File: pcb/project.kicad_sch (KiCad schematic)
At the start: 5 parts, among them J1 USB_B_Micro, U1 RP2040, U2 NCP1117-3.3_SOT223

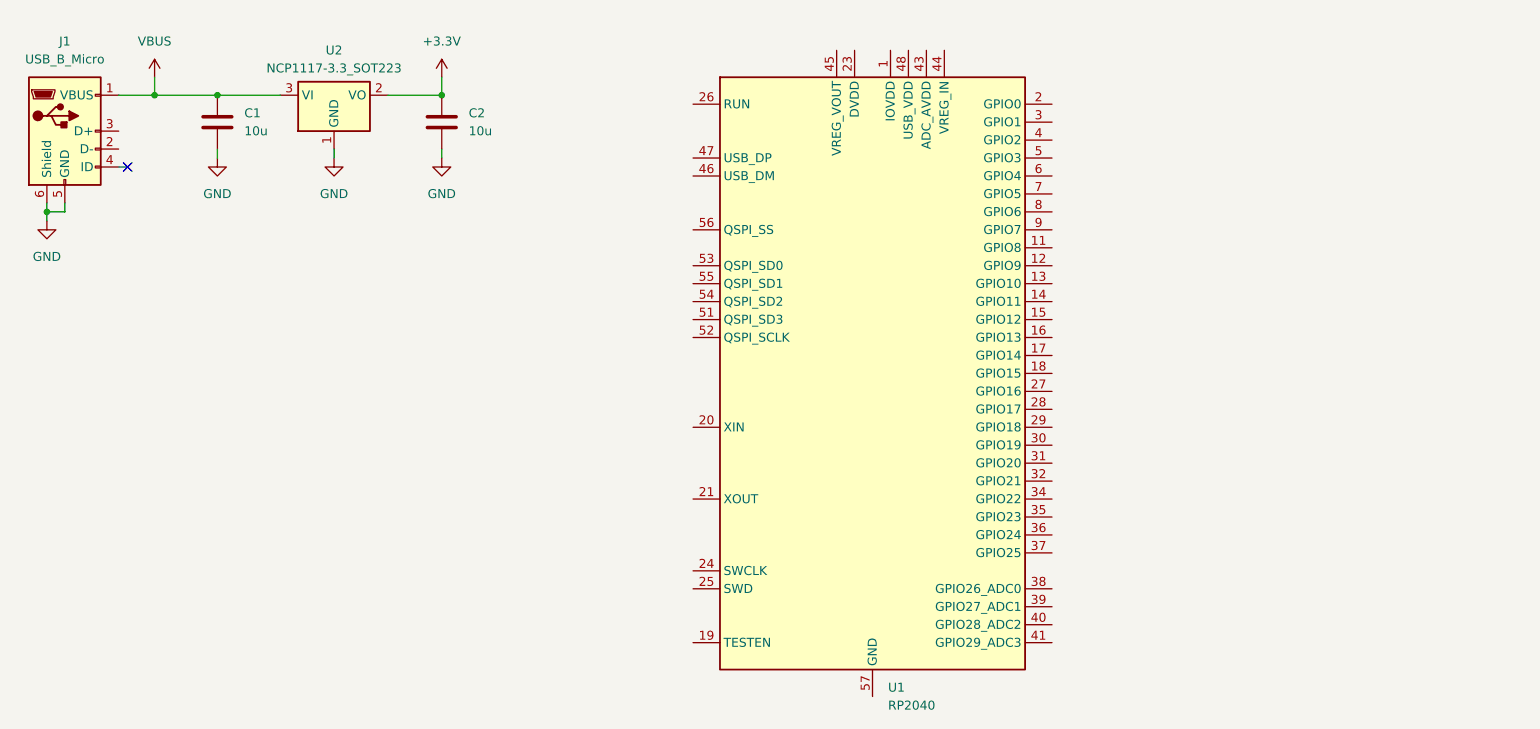
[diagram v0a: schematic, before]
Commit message: Implemented circuit
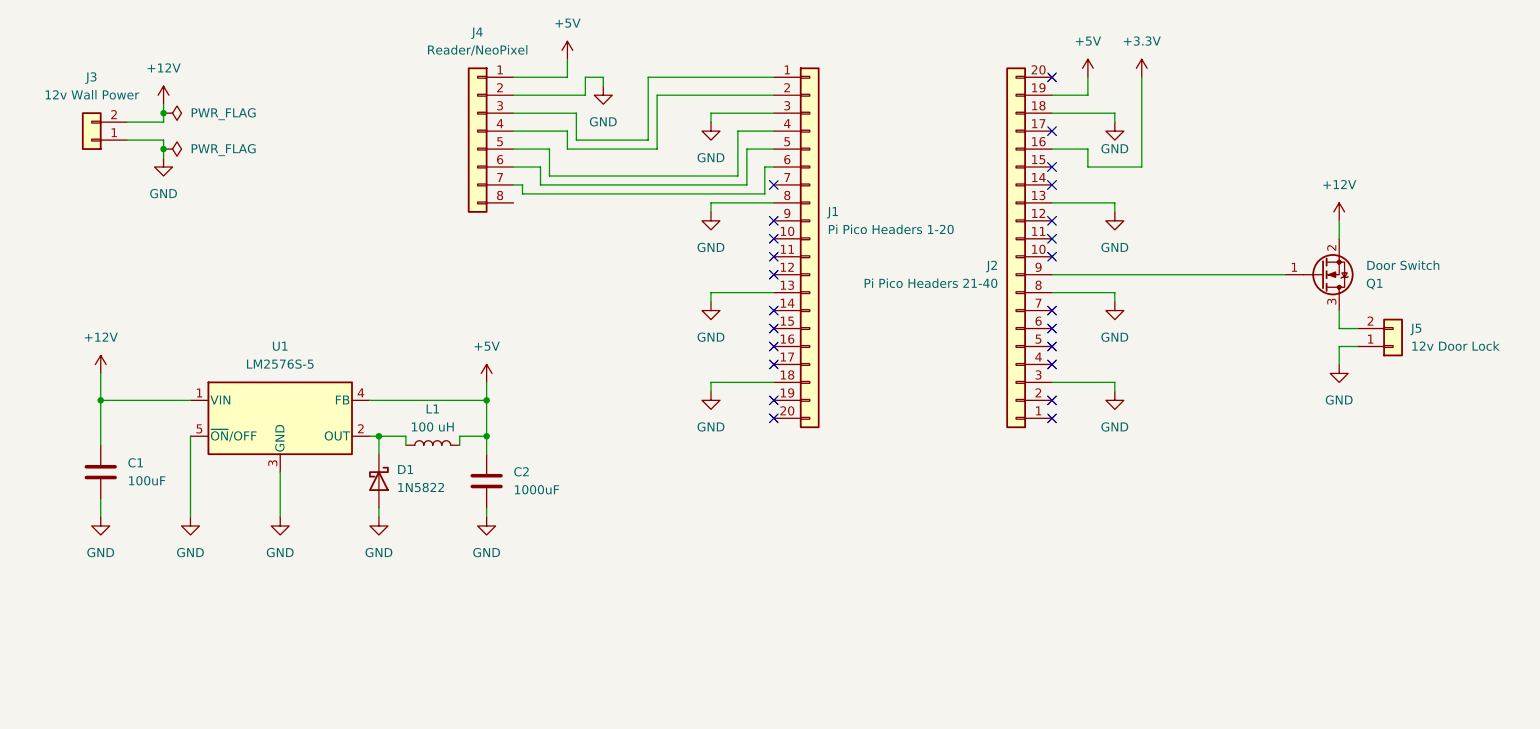
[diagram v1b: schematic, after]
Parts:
- removed J1: USB_B_Micro, symbol Connector:USB_B_Micro
- removed U1: RP2040, Package_DFN_QFN:QFN-56-1EP_7x7mm_P0.4mm_EP3.2x3.2mm, symbol MCU_RaspberryPi:RP2040
- removed U2: NCP1117-3.3_SOT223, Package_TO_SOT_SMD:SOT-223-3_TabPin2, symbol Regulator_Linear:NCP1117-3.3_SOT223
- added D1: 1N5822, Diode_SMD:D_0603_1608Metric, symbol Diode:1N5822
- added J1: Pi Pico Headers 1-20, Connector_PinSocket_2.54mm:PinSocket_1x20_P2.54mm_Vertical, symbol Connector_Generic:Conn_01x20
- added J2: Pi Pico Headers 21-40, Connector_PinSocket_2.54mm:PinSocket_1x20_P2.54mm_Vertical, symbol Connector_Generic:Conn_01x20
- added J3: 12v Wall Power, Connector_JST:JST_PH_B2B-PH-K_1x02_P2.00mm_Vertical, symbol Connector_Generic:Conn_01x02
- added J4: Reader/NeoPixel, Connector_JST:JST_PH_B8B-PH-K_1x08_P2.00mm_Vertical, symbol Connector_Generic:Conn_01x08
- added J5: 12v Door Lock, Connector_JST:JST_PH_B2B-PH-K_1x02_P2.00mm_Vertical, symbol Connector_Generic:Conn_01x02
- added L1: 100 uH, Inductor_SMD:L_0603_1608Metric, symbol Device:L
- added Q1: Door Switch, Package_TO_SOT_SMD:SOT-23, symbol Transistor_FET:DMN2040U
- added U1: LM2576S-5, Package_TO_SOT_SMD:TO-263-5_TabPin3, symbol Regulator_Switching:LM2576S-5
- C1: value 10u -> 100uF; footprint (none) -> Capacitor_SMD:C_0603_1608Metric
- C2: value 10u -> 1000uF; footprint (none) -> Capacitor_SMD:C_0603_1608Metric
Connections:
- net +3.3V: now also J2.16 (Pin_16); no longer C2.1
- net GND: now also D1.2 (A), J1.13 (Pin_13), J1.18 (Pin_18), J1.3 (Pin_3), J1.8 (Pin_8), J2.13 (Pin_13), J2.18 (Pin_18), J2.3 (Pin_3), J2.8 (Pin_8), J3.1 (Pin_1), J4.2 (Pin_2), J5.1 (Pin_1), U1.3 (GND), U1.5 (~{ON}/OFF)
- net VBUS renamed +12V
- net +12V: now also J3.2 (Pin_2), Q1.2 (S), U1.1 (VIN)
- new net: J1.1 (Pin_1), J4.3 (Pin_3)
- new net: J1.2 (Pin_2), J4.4 (Pin_4)
- new net: J1.4 (Pin_4), J4.5 (Pin_5)
- new net: J1.5 (Pin_5), J4.6 (Pin_6)
- new net: J1.6 (Pin_6), J4.7 (Pin_7)
- new net: J2.9 (Pin_9), Q1.1 (G)
- new net: J5.2 (Pin_2), Q1.3 (D)
- new net: D1.1 (K), L1.1, U1.2 (OUT)
- new net +5V: C2.1, J2.19 (Pin_19), J4.1 (Pin_1), L1.2, U1.4 (FB)
- no-connect marks 1 -> 24
